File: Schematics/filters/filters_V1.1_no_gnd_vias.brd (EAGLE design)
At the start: 100.6 x 47.9 mm, 110 parts, among them IC1 NE5532N, IC2 NE5532N, IC3 NE5532N, IC4 NE5532N, IC5 NE5532N, IC6 NE5532N, IC7 NE5532N, J1 3_PIN_AMPCONN, J2 3_PIN_AMPCONN, J3 3_PIN_AMPCONN

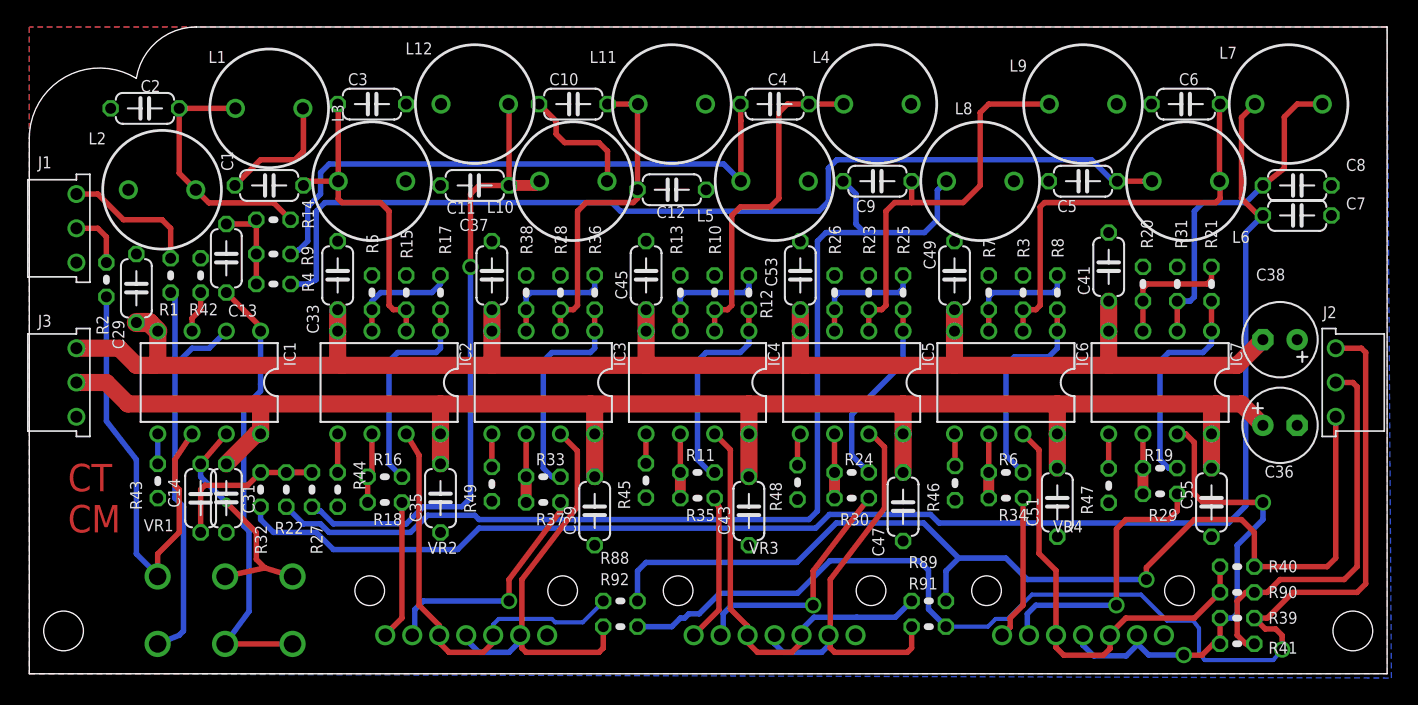
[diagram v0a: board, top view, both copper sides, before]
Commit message: newest gerbers
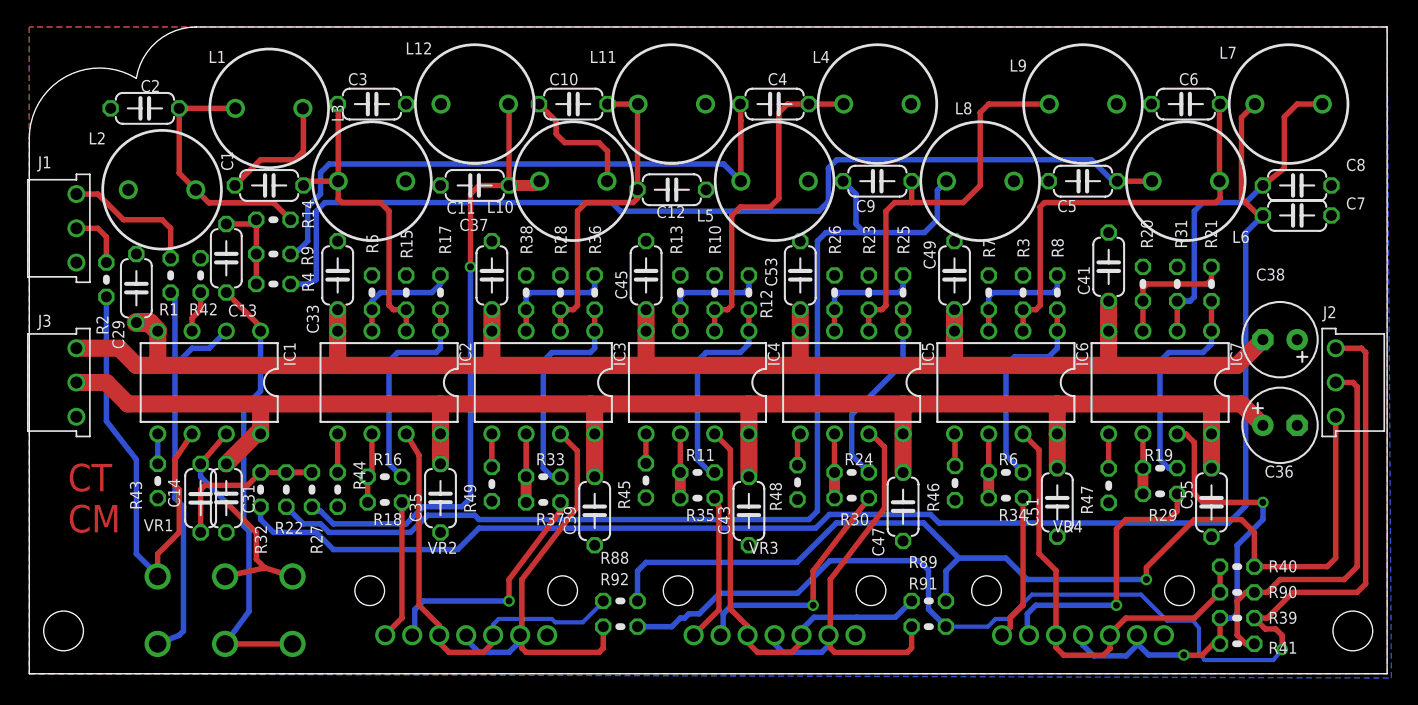
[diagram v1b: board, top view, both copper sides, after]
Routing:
- net N$5: vias 1 -> 0
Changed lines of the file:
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@@
 <wire x1="12.7" y1="15.5575" x2="12.7" y2="14.605" width="0.4064" layer="16"/>
 <wire x1="12.7" y1="14.605" x2="14.605" y2="12.7" width="0.4064" layer="16"/>
-<via x="14.605" y="12.7" extent="1-16" drill="0.381"/>
+<wire x1="14.605" y1="12.7" x2="14.605" y2="12.7" width="0" layer="19" extent="1-16"/>
 <wire x1="14.605" y1="12.7" x2="16.8275" y2="10.4775" width="0.4064" layer="1"/>
 <wire x1="16.8275" y1="10.4775" x2="16.8275" y2="8.4826125" width="0.4064" layer="1"/>
@@
 <contactref element="L12" pad="2"/>
 <contactref element="C11" pad="1"/>
-<via x="32.7025" y="30.1625" extent="1-16" drill="0.8128"/>
+<via x="32.7025" y="30.1625" extent="1-16" drill="0.508"/>
 <wire x1="32.7025" y1="30.1625" x2="32.7025" y2="35.56" width="0.4064" layer="1"/>
 <wire x1="35.56" y1="36.195" x2="37.505" y2="36.195" width="0.8128" layer="1"/>
@@
 <contactref element="R29" pad="2"/>
 <contactref element="VR4" pad="1'"/>
-<via x="80.5815" y="5.08" extent="1-16" drill="0.8128"/>
+<via x="80.5815" y="5.08" extent="1-16" drill="0.508"/>
 <wire x1="80.5815" y1="5.08" x2="74.6125" y2="5.08" width="0.4064" layer="16"/>
 <wire x1="74.6125" y1="5.08" x2="73.9775" y2="4.445" width="0.4064" layer="16"/>
@@
 <contactref element="VR3" pad="1'"/>
 <wire x1="58.1025" y1="7.62" x2="58.1025" y2="5.08" width="0.4064" layer="1"/>
-<via x="58.1025" y="5.08" extent="1-16" drill="0.8128"/>
+<via x="58.1025" y="5.08" extent="1-16" drill="0.508"/>
 <wire x1="58.1025" y1="5.08" x2="52.07" y2="5.08" width="0.4064" layer="16"/>
 <wire x1="52.07" y1="5.08" x2="51.435" y2="4.445" width="0.4064" layer="16"/>
@@
 <contactref element="VR2" pad="1'"/>
 <wire x1="35.56" y1="6.985" x2="35.56" y2="5.3975" width="0.4064" layer="1"/>
-<via x="35.56" y="5.3975" extent="1-16" drill="0.8128"/>
+<via x="35.56" y="5.3975" extent="1-16" drill="0.508"/>
 <wire x1="35.56" y1="5.3975" x2="29.21" y2="5.3975" width="0.4064" layer="16"/>
 <wire x1="29.21" y1="5.3975" x2="28.575" y2="4.7625" width="0.4064" layer="16"/>
@@
 <wire x1="96.2025" y1="7.9375" x2="90.805" y2="7.9375" width="0.4064" layer="1"/>
 <wire x1="90.805" y1="7.9375" x2="90.805" y2="10.4775" width="0.4064" layer="1"/>
-<via x="82.804" y="6.985" extent="1-16" drill="0.8128"/>
+<via x="82.804" y="6.985" extent="1-16" drill="0.508"/>
 <wire x1="82.804" y1="6.985" x2="73.9775" y2="6.985" width="0.4064" layer="16"/>
 <wire x1="73.9775" y1="6.985" x2="72.39" y2="8.5725" width="0.4064" layer="16"/>
@@
 <wire x1="86.27411875" y1="3.936628125" x2="86.70560625" y2="3.378140625" width="0.3048" layer="16"/>
 <wire x1="86.70560625" y1="3.378140625" x2="86.70560625" y2="1.55939375" width="0.3048" layer="16"/>
-<via x="92.867840625" y="1.79724375" extent="1-16" drill="0.8128"/>
+<via x="92.867840625" y="1.79724375" extent="1-16" drill="0.508"/>
 <wire x1="92.867840625" y1="1.79724375" x2="92.867840625" y2="2.8362375" width="0.4064" layer="1"/>
 <wire x1="92.867840625" y1="2.8362375" x2="92.381596875" y2="3.32248125" width="0.4064" layer="1"/>
@@
 <wire x1="86.919915625" y1="1.375271875" x2="85.59364375" y2="1.375271875" width="0.4064" layer="1"/>
 <wire x1="85.59364375" y1="1.375271875" x2="85.5774625" y2="1.391453125" width="0.4064" layer="1"/>
-<via x="85.5774625" y="1.391453125" extent="1-16" drill="0.8128"/>
+<via x="85.5774625" y="1.391453125" extent="1-16" drill="0.508"/>
 <wire x1="85.5774625" y1="1.391453125" x2="82.973725" y2="1.391453125" width="0.4064" layer="16"/>
 <wire x1="82.973725" y1="1.391453125" x2="82.08384375" y2="2.281334375" width="0.4064" layer="16"/>
@@
 <wire x1="86.36" y1="13.335" x2="86.995" y2="12.7" width="0.4064" layer="1"/>
 <wire x1="86.995" y1="12.7" x2="91.44" y2="12.7" width="0.4064" layer="1"/>
-<via x="91.44" y="12.7" extent="1-16" drill="0.8128"/>
+<via x="91.44" y="12.7" extent="1-16" drill="0.508"/>
 <wire x1="91.44" y1="12.7" x2="91.44" y2="11.43" width="0.4064" layer="16"/>
 <wire x1="91.44" y1="11.43" x2="89.535" y2="9.525" width="0.4064" layer="16"/>
